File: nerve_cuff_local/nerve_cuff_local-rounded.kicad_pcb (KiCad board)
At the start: 2 copper layers, 4.4 x 5.3 mm, 2 parts

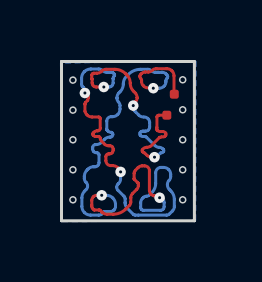
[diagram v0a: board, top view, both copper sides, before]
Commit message: updating constraints, xy board
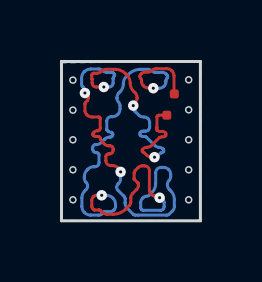
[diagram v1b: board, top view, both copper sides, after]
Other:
- board size 4.4 x 5.3 mm -> 4.6 x 5.3 mm
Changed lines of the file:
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@@
   )
   (footprint "nerve_cuff_pads:small_pad_nerve_cuff" (layer "F.Cu")
-    (at 130.74 65.48)
+    (at 130.74 65.47)
     (descr "Wire Pad, Square, SMD Pad,  1mm x 2mm,")
     (tags "MesurementPoint Square SMDPad 1mmx2mm ")
@@
     (pad "1" smd roundrect (at 0 0) (size 0.3 0.3) (layers "F.Cu" "F.Paste" "F.Mask") (roundrect_rratio 0.25))
   )
-  (gr_circle (center 131.02 68) (end 131.12 68)
-    (stroke (width 0.05) (type default)) (fill none) (layer "Edge.Cuts"))
-  (gr_line (start 126.98 64.39) (end 131.41 64.39)
+  (gr_circle (center 131.22 68) (end 131.32 68)
+    (stroke (width 0.05) (type default)) (fill none) (layer "Edge.Cuts"))
+  (gr_line (start 126.98 64.39) (end 131.61 64.39)
     (stroke (width 0.1) (type default)) (layer "Edge.Cuts"))
-  (gr_line (start 131.41 64.39) (end 131.41 69.7)
+  (gr_line (start 131.61 64.39) (end 131.61 69.7)
     (stroke (width 0.1) (type default)) (layer "Edge.Cuts"))
   (gr_circle (center 127.36 69) (end 127.46 69)
@@
   (gr_line (start 126.98 64.39) (end 126.98 69.7)
     (stroke (width 0.1) (type default)) (layer "Edge.Cuts"))
-  (gr_circle (center 131.02 69) (end 131.12 69)
-    (stroke (width 0.05) (type default)) (fill none) (layer "Edge.Cuts"))
-  (gr_circle (center 131.02 67) (end 131.12 67)
+  (gr_circle (center 131.22 69) (end 131.32 69)
+    (stroke (width 0.05) (type default)) (fill none) (layer "Edge.Cuts"))
+  (gr_circle (center 131.22 67) (end 131.32 67)
     (stroke (width 0.05) (type default)) (fill none) (layer "Edge.Cuts"))
   (gr_circle (center 127.36 67) (end 127.46 67)
@@
   (gr_circle (center 127.36 68) (end 127.46 68)
     (stroke (width 0.05) (type default)) (fill none) (layer "Edge.Cuts"))
-  (gr_line (start 126.98 69.7) (end 131.41 69.7)
+  (gr_line (start 126.98 69.7) (end 131.61 69.7)
     (stroke (width 0.1) (type default)) (layer "Edge.Cuts"))
-  (gr_circle (center 131.02 65) (end 131.12 65)
+  (gr_circle (center 131.22 65) (end 131.32 65)
     (stroke (width 0.05) (type default)) (fill none) (layer "Edge.Cuts"))
   (gr_circle (center 127.36 66.01) (end 127.46 66.01)
     (stroke (width 0.05) (type default)) (fill none) (layer "Edge.Cuts"))
-  (gr_circle (center 131.02 66) (end 131.12 66)
+  (gr_circle (center 131.22 66) (end 131.32 66)
     (stroke (width 0.05) (type default)) (fill none) (layer "Edge.Cuts"))
   (dimension (type aligned) (layer "F.SilkS")
@@
     (height -6.07)
     (gr_text "5.3000 mm" (at 136.12 67.05 90) (layer "F.SilkS")
-      (effects (font (size 1 1) (thickness 0.15)))
-    )
-    (format (prefix "") (suffix "") (units 3) (units_format 1) (precision 4))
-    (style (thickness 0.15) (arrow_length 1.27) (text_position_mode 0) (extension_height 0.58642) (extension_offset 0.5) keep_text_aligned)
-  )
-  (dimension (type aligned) (layer "F.SilkS")
-    (pts (xy 127.36 69.49) (xy 131.02 69.49))
-    (height 3.46)
-    (gr_text "3.6600 mm" (at 129.19 71.8) (layer "F.SilkS")
       (effects (font (size 1 1) (thickness 0.15)))
     )
@@
         (xy 126.99 64.36)
         (xy 126.99 69.7)
-        (xy 131.43 69.69)
-        (xy 131.43 64.39)
+        (xy 131.62 69.71)
+        (xy 131.62 64.38)
       )
     )
@@
       (pts
         (xy 126.95 64.44)
-        (xy 126.999829 69.730898)
-        (xy 131.449829 69.690898)
-        (xy 131.459829 64.370898)
+        (xy 126.97 69.69)
+        (xy 131.619829 69.690898)
+        (xy 131.629829 64.370898)
       )
     )
